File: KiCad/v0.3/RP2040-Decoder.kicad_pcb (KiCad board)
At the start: 2 copper layers, 23.5 x 20 mm, 56 parts, among them J1 T0, J10 2, J11 3, J12 4, J13 5, J14 +V, J15 M_OUT_B, J16 M_OUT_A, J17 GND, J18 SWCLK, J19 SWDIO, J2 T1, J20 RUN, J3 0, J4 1, J5 2, J6 3, J7 +3V3, J8 0, J9 1, Q1 T2N7002BK, Q2 T2N7002BK, Q3 T2N7002BK, Q4 T2N7002BK, Q5 T2N7002BK, U1 PJ75AL33SA, U2 BDR6133, U3 W25Q64JVSSIQ, U4 RP2040, Y1 X322512MSB4SI

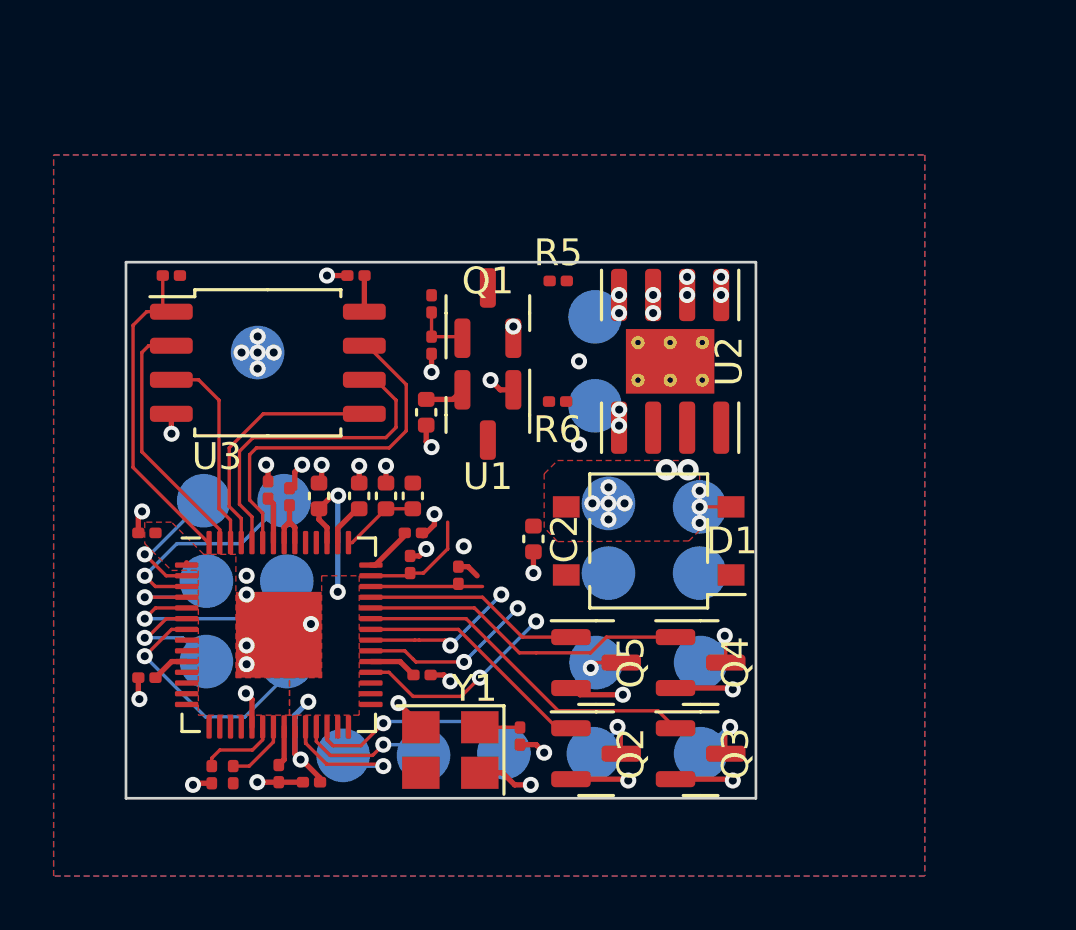
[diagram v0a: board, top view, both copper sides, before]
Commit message: changes
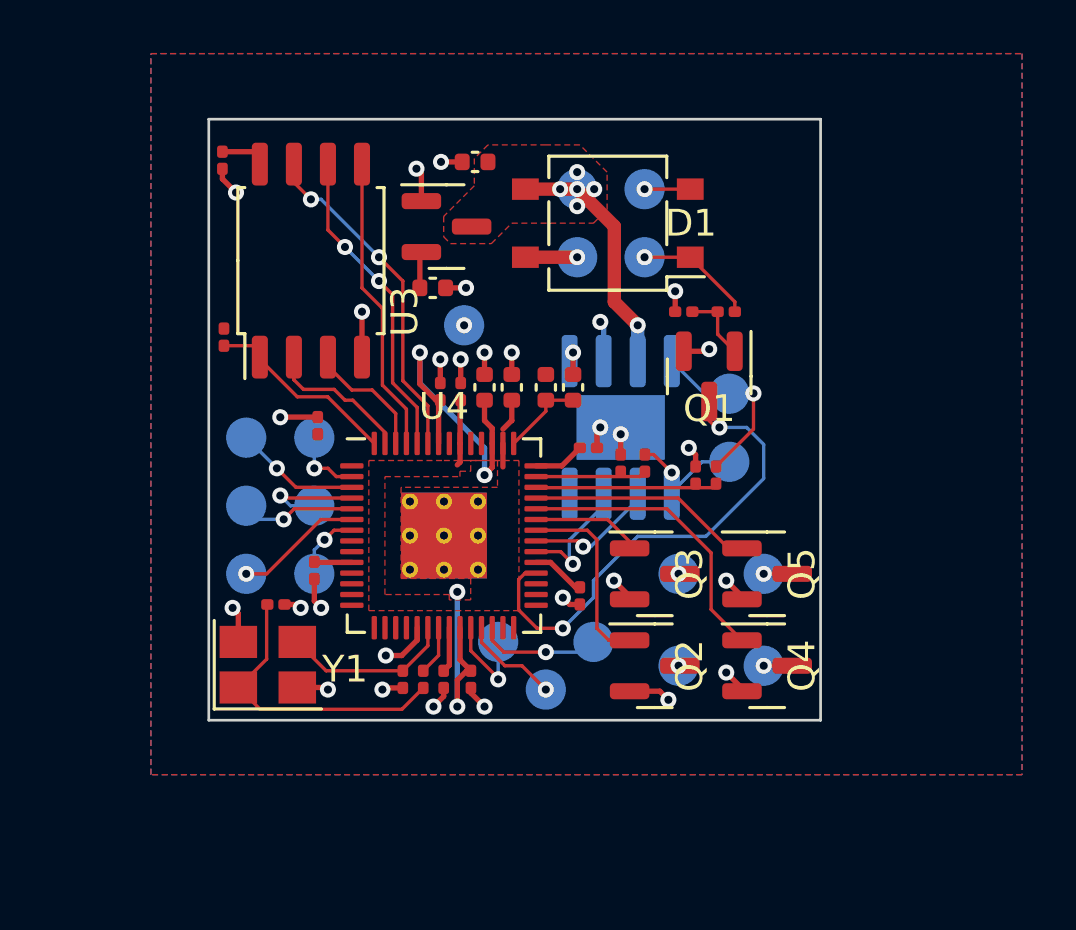
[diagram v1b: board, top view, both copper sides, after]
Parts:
- J1, J10, J11, J12, J13, J14, J15, J16, J17, J18, J19, J2, J20, J3, J4, J5, J6, J7, J8, J9: footprint TestPoint:TestPoint_Pad_D2.0mm -> TestPoint:TestPoint_Pad_D1.5mm
- U2: footprint RP2040-Decoder_Additional_Footprints:SOIC-8-1EP_3.9x4.9mm_P1.27mm_EP2.41x3.3mm_ThermalVias -> Package_SO:SOIC-8-1EP_3.9x4.9mm_P1.27mm_EP2.41x3.3mm; moved to B.Cu
- U4: footprint RP2040-Decoder_Additional_Footprints:QFN-56-1EP_7x7mm_P0.4mm_EP3.2x3.2mm -> User:QFN-56-1EP_7x7mm_P0.4mm_EP3.2x3.2mm_BigThermalVias
- moved C2 14.2 mm to (150.5, 86.4), turned to 180 degrees
- moved J2 12.0 mm to (156.8, 87.4)
- moved J1 12.0 mm to (156.8, 89.9)
- moved D1 12.0 mm to (155.5, 88.6)
- moved J17 11.8 mm to (154.3, 89.9)
- moved J14 11.8 mm to (154.3, 87.4)
- moved R1 11.0 mm to (159.9, 91.9), turned to 0 degrees
- moved C17 10.3 mm to (143.1, 102.9), turned to 0 degrees
- moved R7 9.61 mm to (158.8, 98.0)
- moved R2 9.49 mm to (158.3, 91.9), turned to 0 degrees
- moved R5 9.33 mm to (159.5, 98.0), turned to 90 degrees
- moved R8 8.72 mm to (156.0, 97.6)
- moved Q1 8.59 mm to (159.3, 94.4), turned to -90 degrees
- moved C14 8.07 mm to (154.2, 94.8)
- moved C16 7.97 mm to (147.8, 105.7)
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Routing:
- net /GPIO21: track 7.70 -> 18.4 mm
- net Net-(C17-Pad1): track 1.50 -> 11.1 mm
- net +V: track 0.00 -> 9.28 mm, vias 9 -> 6
- net /GPIO25: track 13.4 -> 4.19 mm
- net +1V1: track 12.5 -> 20.0 mm
- net /MOTOR_OUT_A: track 0.00 -> 6.85 mm, vias 2 -> 1
- net /GPIO5: track 9.36 -> 2.59 mm
- net /QSPI_SS: track 12.2 -> 6.91 mm
- net Net-(J1-Pin_1): track 0.00 -> 4.43 mm, vias 0 -> 1
- net /QSPI_SD1: track 9.50 -> 5.47 mm
- net /RUN: track 8.03 -> 4.06 mm
- net /MOTOR_OUT_B: track 0.00 -> 3.90 mm, vias 2 -> 1
- net /XIN: track 2.96 -> 6.38 mm
- net /GPIO1: track 8.09 -> 4.71 mm
- net /GPIO3: track 7.61 -> 4.31 mm
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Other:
- board size 23.5 x 20 mm -> 22.8 x 22.4 mm
